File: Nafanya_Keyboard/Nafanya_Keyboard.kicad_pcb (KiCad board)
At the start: 2 copper layers, 192 x 101 mm, 57 parts, among them J1 Speaker/Reset/Power, J2 Columns, J3 Rows, J4 Faceplate GND, SW1 1, SW10 0, SW11 Q, SW12 W, SW13 E, SW14 R, SW15 T, SW16 Y, SW17 U, SW18 I, SW19 O, SW2 2, SW20 P, SW21 A, SW22 S, SW23 D, SW24 F, SW25 G, SW26 H, SW27 J, SW28 K, SW29 L, SW3 3, SW30 ENTER, SW31 CAPS_SHIFT, SW32 Z, SW33 X, SW34 C, SW35 V, SW36 B, SW37 N, SW38 M, SW39 SYMBOL_SHIFT, SW4 4, SW40 BREAK_SPACE, SW41 RESET, SW5 5, SW6 6, SW7 7, SW8 8, SW9 9

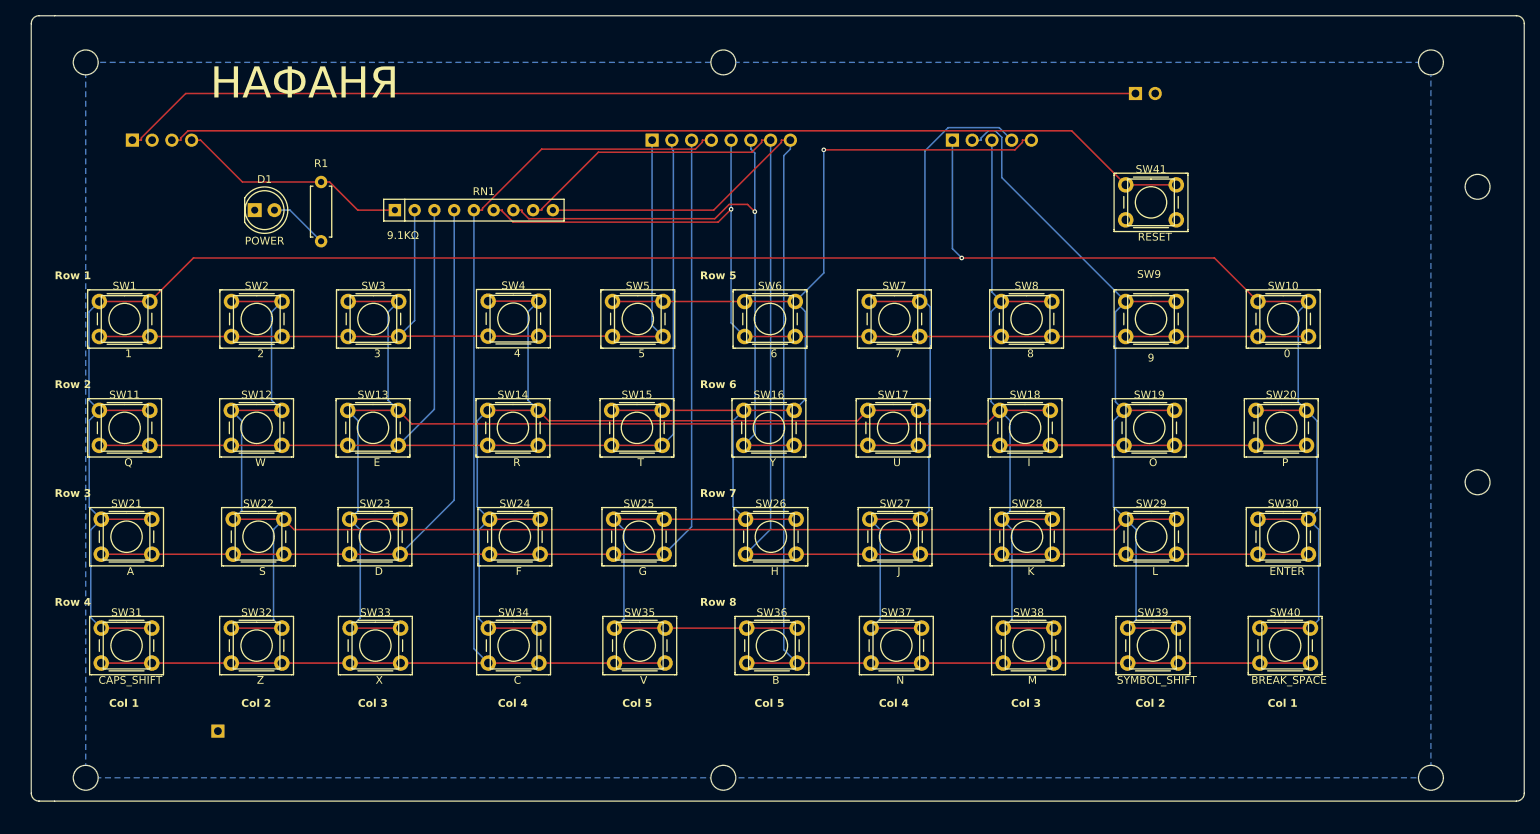
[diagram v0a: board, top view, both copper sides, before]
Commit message: Finalised layout
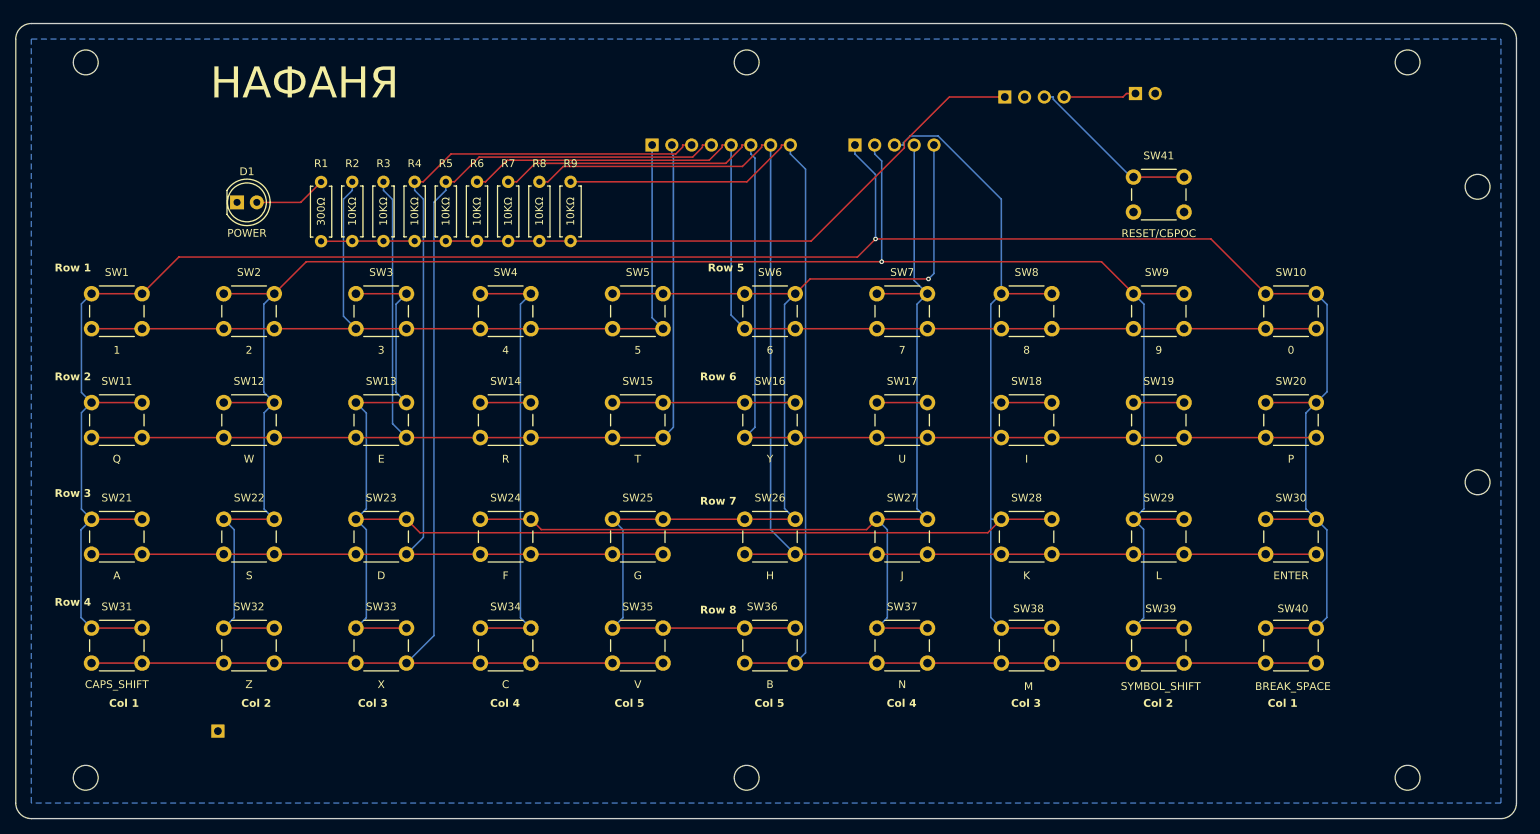
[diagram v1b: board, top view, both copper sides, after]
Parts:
- removed RN1: 9.1KΩ, Resistor_THT:R_Array_SIP9
- added R2: 10KΩ, Resistor_THT:R_Axial_DIN0207_L6.3mm_D2.5mm_P7.62mm_Horizontal, F.Cu at (95.3, 79.0)
- added R3: 10KΩ, Resistor_THT:R_Axial_DIN0207_L6.3mm_D2.5mm_P7.62mm_Horizontal, F.Cu at (99.3, 79.0)
- added R4: 10KΩ, Resistor_THT:R_Axial_DIN0207_L6.3mm_D2.5mm_P7.62mm_Horizontal, F.Cu at (103.3, 79.0)
- added R5: 10KΩ, Resistor_THT:R_Axial_DIN0207_L6.3mm_D2.5mm_P7.62mm_Horizontal, F.Cu at (107.3, 79.0)
- added R6: 10KΩ, Resistor_THT:R_Axial_DIN0207_L6.3mm_D2.5mm_P7.62mm_Horizontal, F.Cu at (111.3, 79.0)
- added R7: 10KΩ, Resistor_THT:R_Axial_DIN0207_L6.3mm_D2.5mm_P7.62mm_Horizontal, F.Cu at (115.3, 79.0)
- added R8: 10KΩ, Resistor_THT:R_Axial_DIN0207_L6.3mm_D2.5mm_P7.62mm_Horizontal, F.Cu at (119.3, 79.0)
- added R9: 10KΩ, Resistor_THT:R_Axial_DIN0207_L6.3mm_D2.5mm_P7.62mm_Horizontal, F.Cu at (123.3, 79.0)
- SW41: value RESET -> RESET/СБРОС
- moved J1 112.3 mm to (179.2, 60.5)
- moved J2 12.6 mm to (159.9, 66.6)
- moved R1 7.62 mm to (91.3, 71.4), turned to -90 degrees
- moved SW30 4.81 mm to (216.0, 117.0)
- moved SW29 4.78 mm to (199.0, 117.0)
- moved SW27 4.74 mm to (166.0, 117.0)
- moved SW20 4.67 mm to (216.0, 102.0)
- moved SW19 4.64 mm to (199.0, 102.0)
- moved SW23 4.64 mm to (99.0, 117.0)
- moved SW17 4.59 mm to (166.0, 102.0)
- moved SW33 4.59 mm to (99.0, 131.0)
- moved SW37 4.59 mm to (166.0, 131.0)
- moved SW39 4.59 mm to (199.0, 131.0)
- moved SW40 4.59 mm to (216.0, 131.0)
- moved SW13 4.48 mm to (99.0, 102.0)
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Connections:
- J1 pad 1: SPEAKER -> +5V
- J1 pad 4: +5V -> SPEAKER
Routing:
- net SPEAKER: track 131.7 -> 9.37 mm
- net RESET: track 132.7 -> 22.4 mm
- net +5V: track 29.9 -> 96.1 mm
- net ROW6: track 161.2 -> 145.2 mm, vias 1 -> 0
- net ROW3: track 174.2 -> 160.5 mm
- net COL5: track 187.8 -> 176.1 mm
- net COL3: track 242.3 -> 253.0 mm
- net COL2: track 284.3 -> 274.1 mm, vias 0 -> 1
- net COL4: track 219.2 -> 210.8 mm
- net ROW4: track 166.1 -> 173.8 mm
- net ROW8: track 175.3 -> 171.9 mm
- net COL1: track 305.2 -> 308.2 mm
- net ROW1: track 115.5 -> 117.7 mm
- net ROW5: track 130.4 -> 132.7 mm, vias 1 -> 0
- net ROW7: track 161.5 -> 159.3 mm
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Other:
- board size 192 x 101 mm -> 193 x 102.2 mm
- board text added: "10мм"
- board text added: "14мм"
- board text added: "17мм"
- board text added: "Принтер Тест"
